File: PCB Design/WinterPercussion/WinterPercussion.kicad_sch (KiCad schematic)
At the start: 2 parts

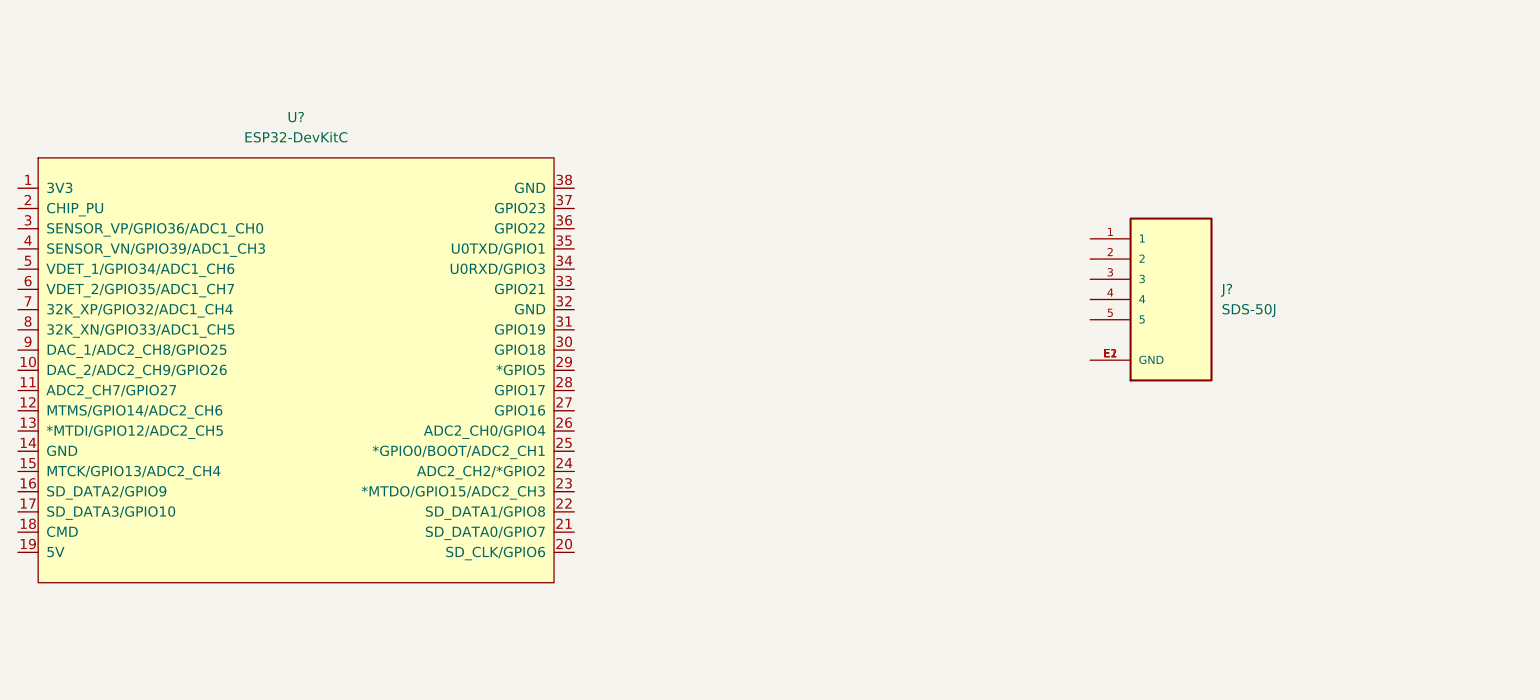
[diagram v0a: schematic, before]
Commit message: Board Design
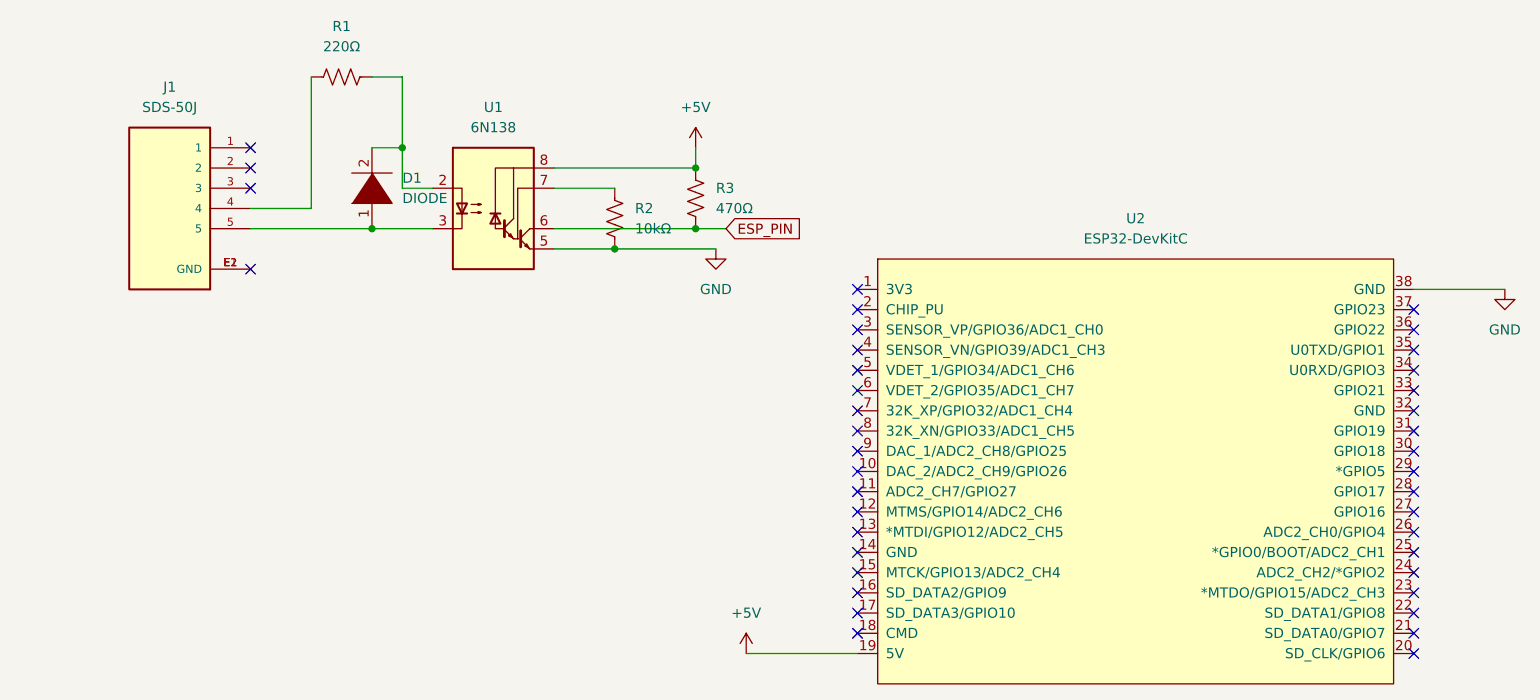
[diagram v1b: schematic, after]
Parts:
- added D1: DIODE, Diode_THT:D_T-1_P5.08mm_Horizontal, symbol pspice:DIODE
- added R1: 220Ω, Resistor_THT:R_Axial_DIN0207_L6.3mm_D2.5mm_P7.62mm_Horizontal, symbol Device:R_US
- added R2: 10kΩ, Resistor_THT:R_Axial_DIN0207_L6.3mm_D2.5mm_P7.62mm_Horizontal, symbol Device:R_US
- added R3: 470Ω, Resistor_THT:R_Axial_DIN0207_L6.3mm_D2.5mm_P7.62mm_Horizontal, symbol Device:R_US
- added U1: 6N138, OptoCoupler:DIP762W50P254L1018H450Q8, symbol Isolator:6N138
- gave numbers to parts that had none: 2
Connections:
- net at J1.4: now also R1.2
- net at J1.5: now also D1.1 (K), U1.3 (C2)
- net +5V: now reaches U2.19 (5V)
- net +5V: now also R3.1, U1.8 (VCC)
- net GND: now reaches U2.38 (GND)
- net GND: now also R2.2, U1.5 (GND)
- new net: D1.2 (A), R1.1, U1.2 (C1)
- new net: R2.1, U1.7 (VO1)
- new net ESP_PIN: R3.2, U1.6 (VO2)
- no-connect marks 0 -> 40
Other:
- moved on the sheet: J1, U2
